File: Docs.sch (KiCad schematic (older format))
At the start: 0 parts

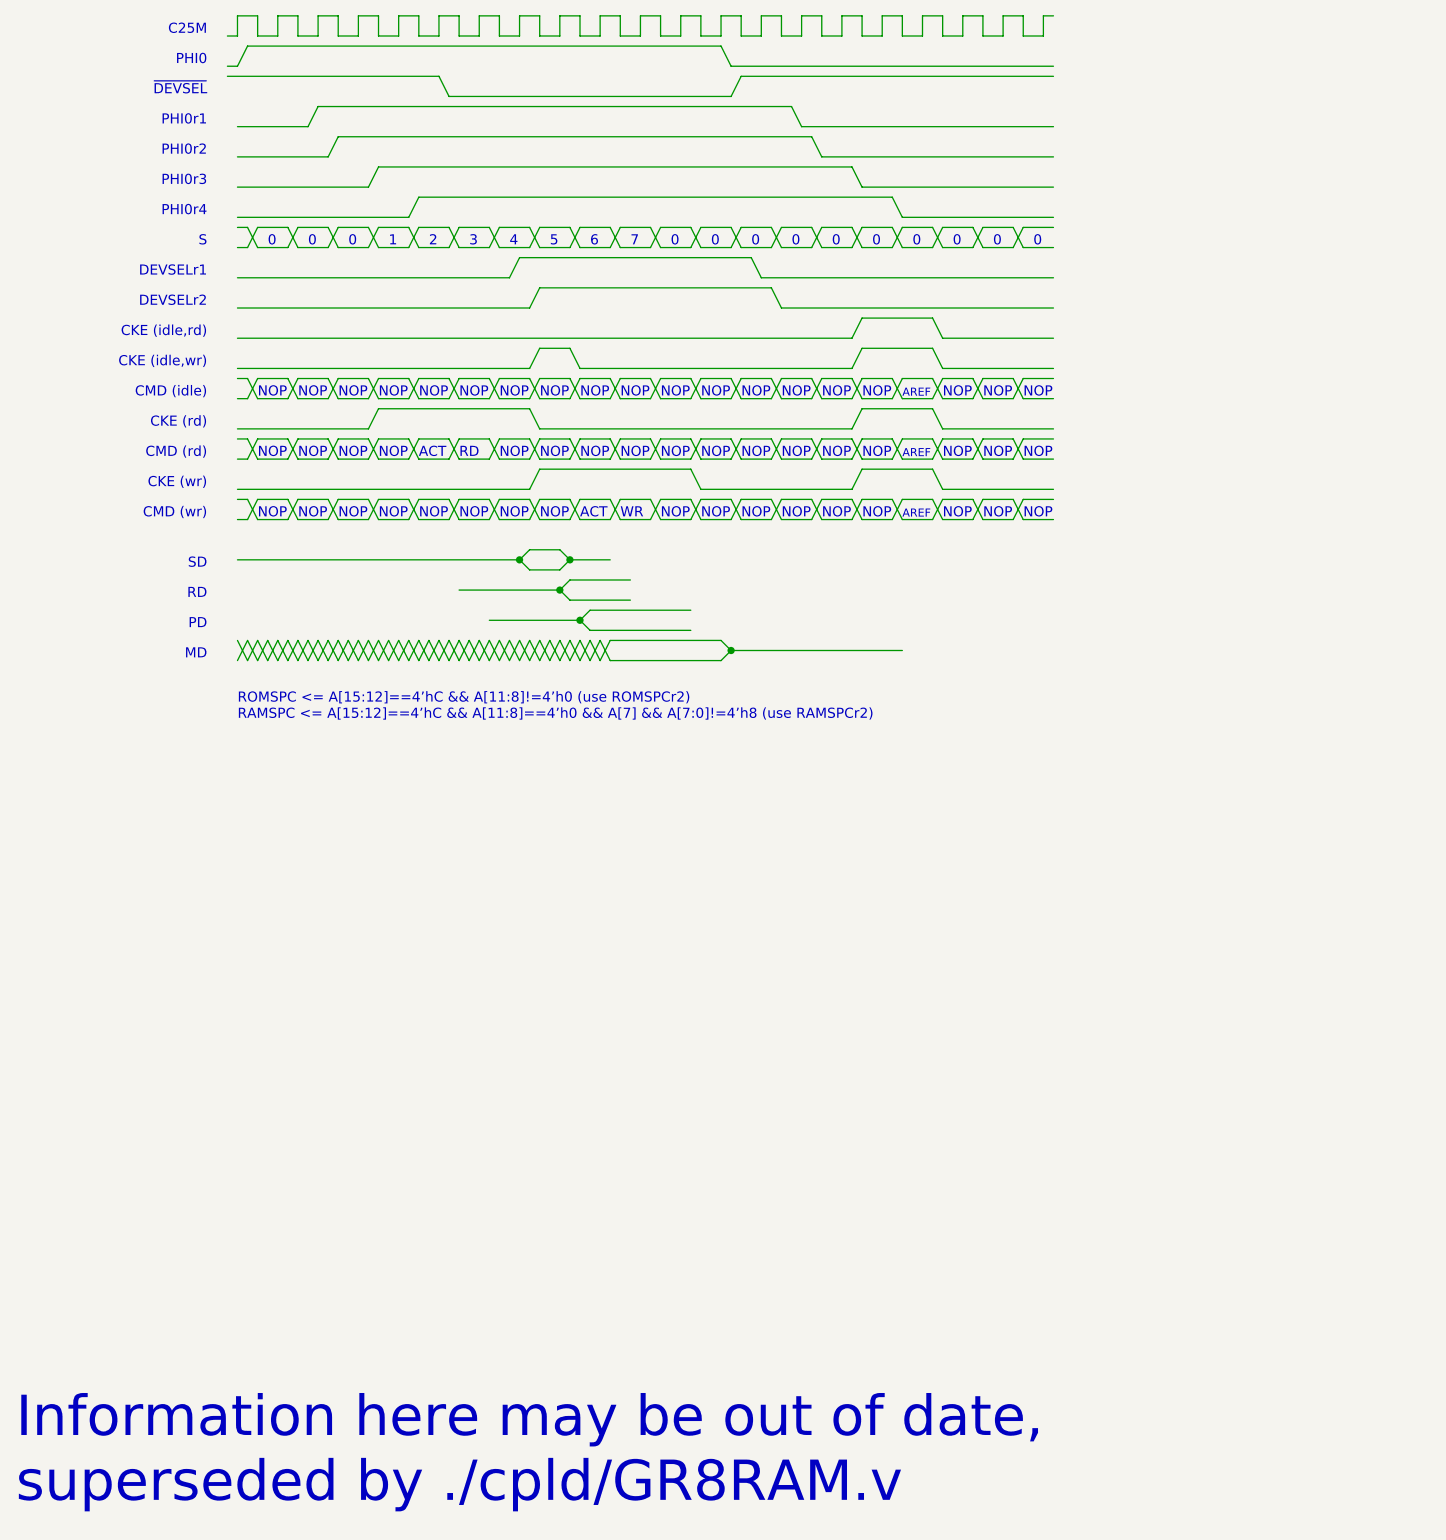
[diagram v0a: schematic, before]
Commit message: idk
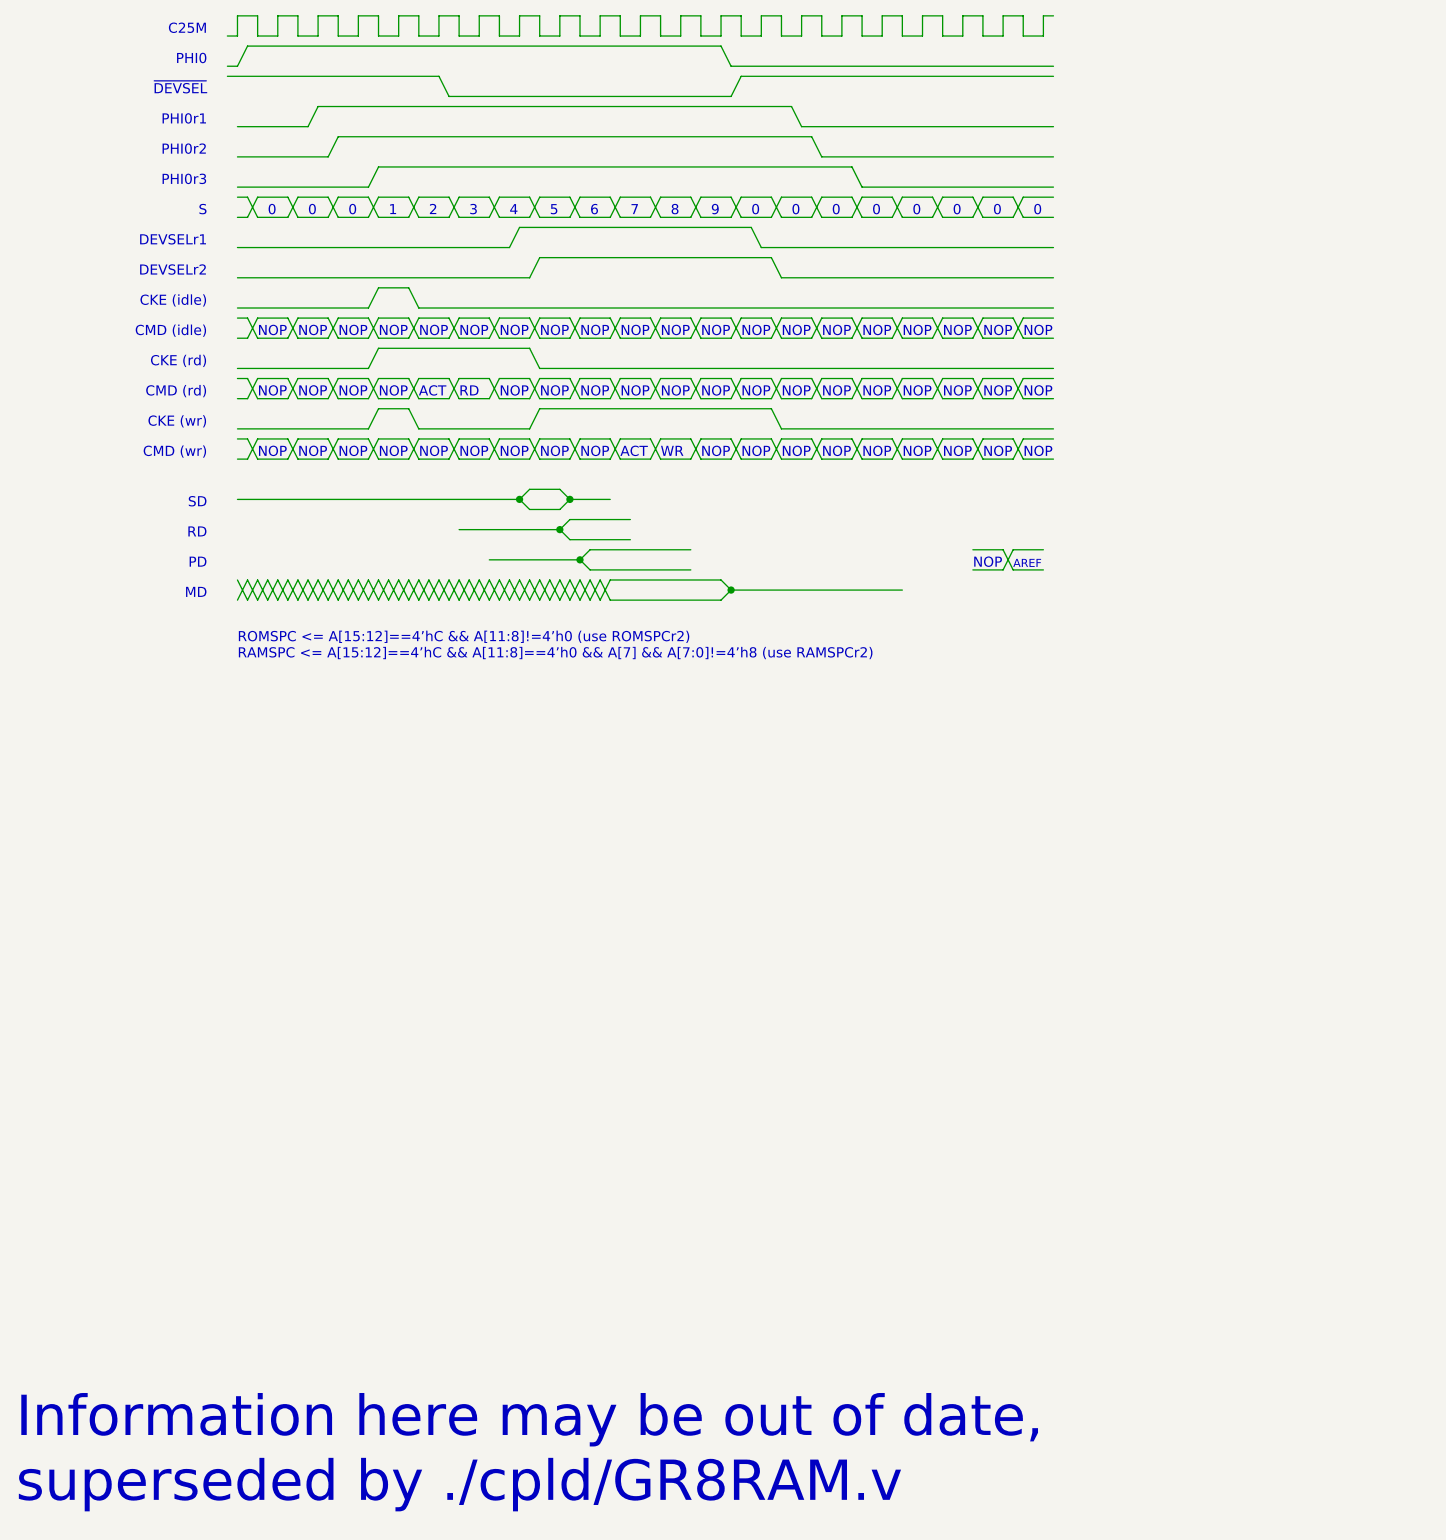
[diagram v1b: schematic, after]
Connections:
- wire segments 580 -> 568
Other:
- note added: "8"
- note added: "9"
- note added: "CKE (idle)"
- note removed: "CKE (idle,rd)"
- note removed: "CKE (idle,wr)"
- note removed: "PHI0r4"
